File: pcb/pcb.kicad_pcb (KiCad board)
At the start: 2 copper layers, 55 x 70 mm, 61 parts, among them J1 SW, J2 HEATER, J3 FAN, J4 BME280, J5 DISPLAY, J6 NTC, J7 POWER, Q1 IRFR9024NTRPBF, Q2 2n3904S-RTK/PS_C18536, Q3 2n3904S-RTK/PS_C18536, Q4 2n3904S-RTK/PS_C18536, SW1 TS-1002S-06026C, SW2 TS-1002S-06026C, SW3 TS-1002S-06026C, U1 STM32F103CBTx, U2 MC34063AD, U3 IRLML5103, Y1 Crystal_GND24

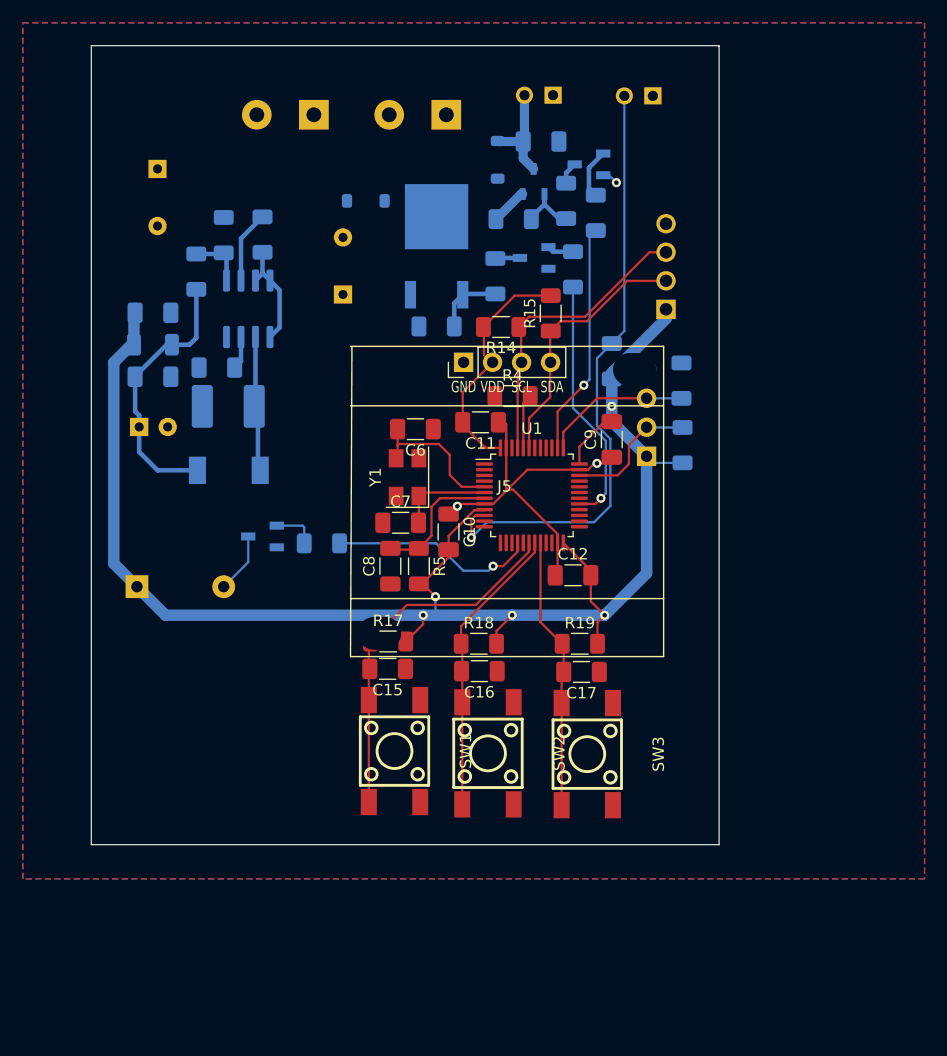
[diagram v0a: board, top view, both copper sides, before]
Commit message: Work with schematics and pcb. update *.ioc files at project.
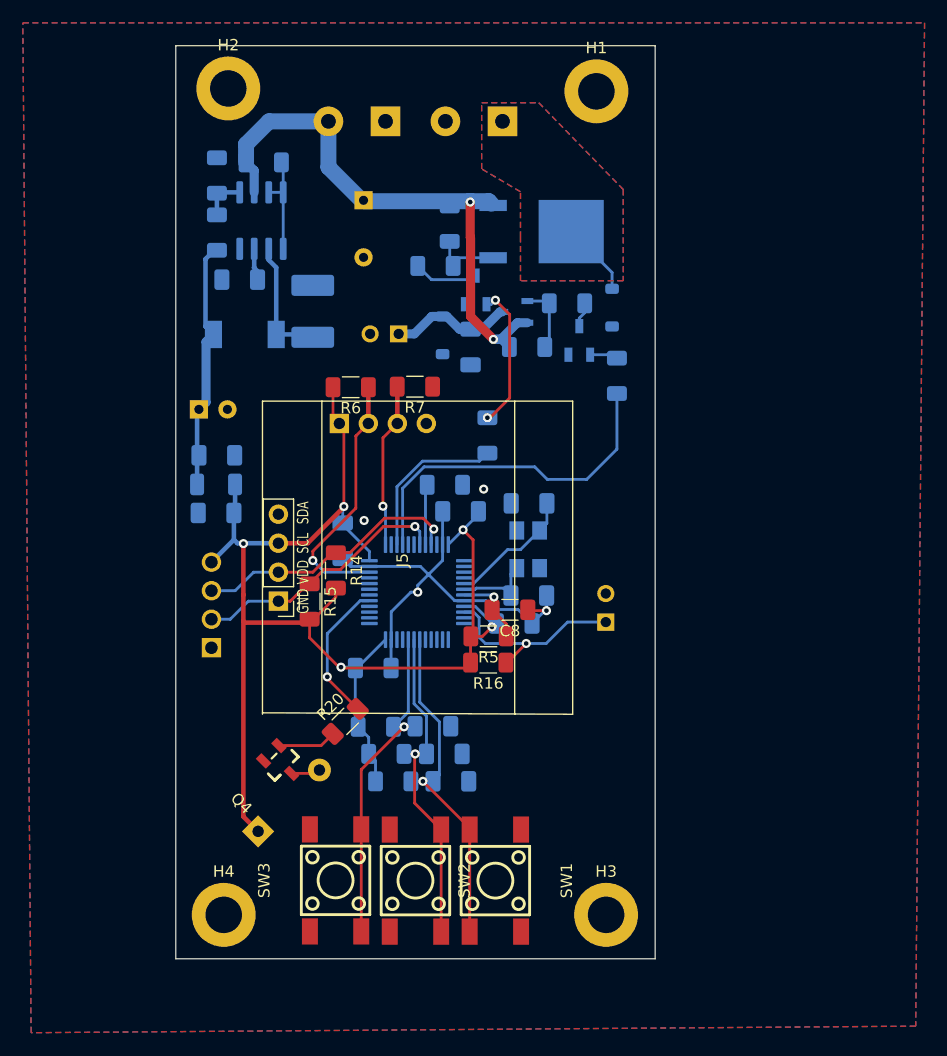
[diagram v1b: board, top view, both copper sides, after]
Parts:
- removed C13: 100uf, Capacitor_THT:CP_Radial_D8.0mm_P5.00mm
- added H1: MountingHole, MountingHole:MountingHole_3.2mm_M3_DIN965_Pad, F.Cu at (94.2, 54.0)
- added H2: MountingHole, MountingHole:MountingHole_3.2mm_M3_DIN965_Pad, F.Cu at (62.0, 53.8)
- added H3: MountingHole, MountingHole:MountingHole_3.2mm_M3_DIN965_Pad, F.Cu at (95.1, 126.2)
- added H4: MountingHole, MountingHole:MountingHole_3.2mm_M3_DIN965_Pad, F.Cu at (61.6, 126.2)
- C10, C11, C12, C15, C16, C17, C6, C7, C9, R17, R18, R19, R4, U1, Y1: moved to B.Cu
- Q4, R16, R20, R6, R7: moved to F.Cu
- moved J4 49.7 mm to (60.5, 99.0)
- moved J6 44.9 mm to (95.1, 99.2), turned to 90 degrees
- moved R15 32.9 mm to (69.1, 98.7), turned to -90 degrees
- moved R6 29.5 mm to (72.7, 79.9), turned to 180 degrees
- moved R16 28.5 mm to (84.8, 104.0), turned to 180 degrees
- moved J1 27.1 mm to (71.7, 83.1), turned to -90 degrees
- moved J5 26.4 mm to (66.4, 94.9), turned to 90 degrees
- moved R14 25.8 mm to (71.4, 96.0), turned to -90 degrees
- moved J3 24.9 mm to (75.7, 75.2)
- moved SW3 24.7 mm to (71.4, 123.1), turned to 90 degrees
- moved BZ1 23.9 mm to (64.6, 118.8), turned to 45 degrees
- moved D1 23.5 mm to (95.6, 73.0), turned to -90 degrees
- moved R7 23.4 mm to (78.3, 79.9), turned to 180 degrees
- moved C12 20.4 mm to (72.0, 93.4), turned to 90 degrees
- moved Q4 19.9 mm to (66.7, 112.9), turned to 135 degrees
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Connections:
- J2 pad 1: GND -> Net-(D1-K)
- J2 pad 2: Net-(D1-K) -> GND
- J3 pad 1: GND -> Net-(D3-K)
- J3 pad 2: Net-(D3-K) -> GND
- J4 pad 1: +3.3V -> GND
- J4 pad 4: GND -> +3.3V
- J6 pad 1: GND -> /NTC
- J6 pad 2: /NTC -> GND
- U1 pad 16: /PWM_BUZZER -> unconnected-(U1-PA6-Pad16)
- U1 pad 29: /PWM_HEATER -> /PWM_BUZZER
- U1 pad 38: /PWM_FAN -> unconnected-(U1-PA15-Pad38)
- U1 pad 39: unconnected-(U1-PB3-Pad39) -> /PWM_HEATER
- U1 pad 40: unconnected-(U1-PB4-Pad40) -> /PWM_FAN
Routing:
- net +24V: track 9.62 -> 50.4 mm, vias 0 -> 2
- net /NTC: track 53.6 -> 17.8 mm
- net +3.3V: track 160.2 -> 125.3 mm
- net /SWDIO: track 11.8 -> 22.6 mm, vias 0 -> 1
- net Net-(Q2-B): track 2.32 -> 12.9 mm, vias 0 -> 2
- net /PWM_FAN: track 20.4 -> 30.9 mm, vias 1 -> 0
- net /PWM_HEATER: track 22.0 -> 14.2 mm, vias 1 -> 0
- net Net-(D1-K): track 0.00 -> 6.49 mm
- net /BTN_RIGHT: track 23.9 -> 29.6 mm, vias 0 -> 1
- net GND: track 34.1 -> 39.6 mm, vias 3 -> 4
- net /PWM_BUZZER: track 18.1 -> 12.6 mm
- net Net-(U1-NRST): track 11.6 -> 6.69 mm, vias 0 -> 1
- net Net-(Q2-C): track 2.17 -> 5.72 mm
- net /BTN_OK: track 26.1 -> 29.0 mm, vias 0 -> 1
- net Net-(BZ1-+): track 5.29 -> 2.58 mm
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- added copper zone on B.Cu, net Net-(D1-K)
- added copper zone on F.Cu, net Net-(D1-K)
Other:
- board size 55 x 70 mm -> 42 x 80 mm
